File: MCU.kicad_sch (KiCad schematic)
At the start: 14 parts, among them U4 ATSAMD21G18A-A, Y1 ABS07-32.768KHZ-T

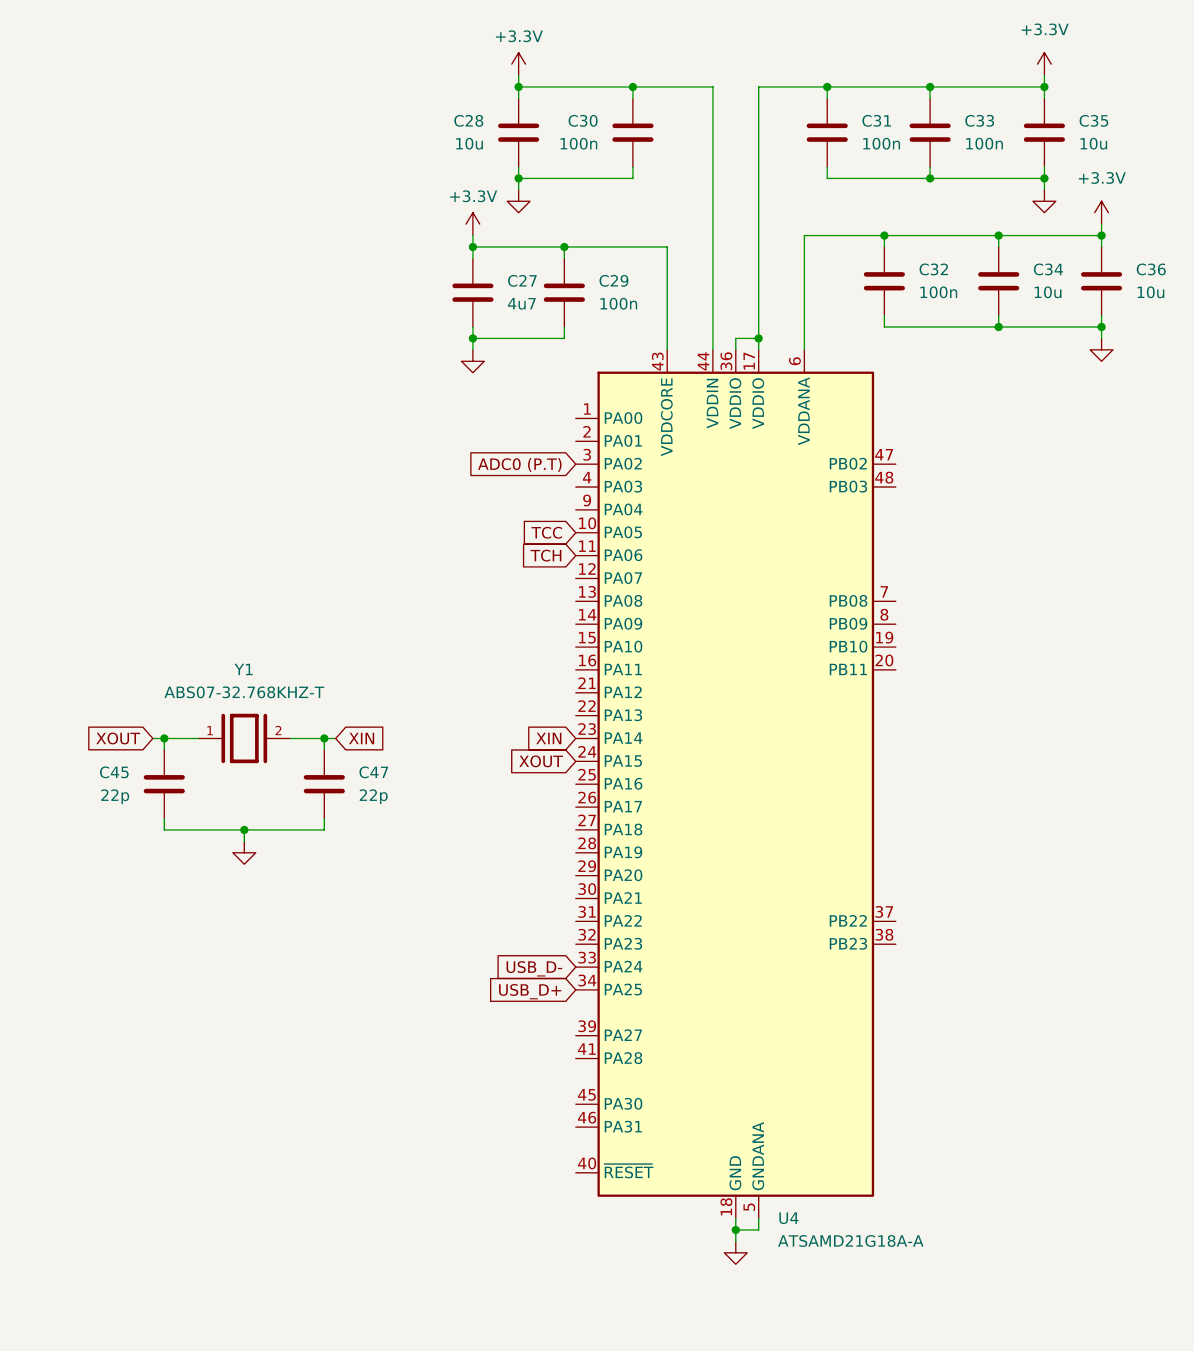
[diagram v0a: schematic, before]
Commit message: Added changes to pass ERC check
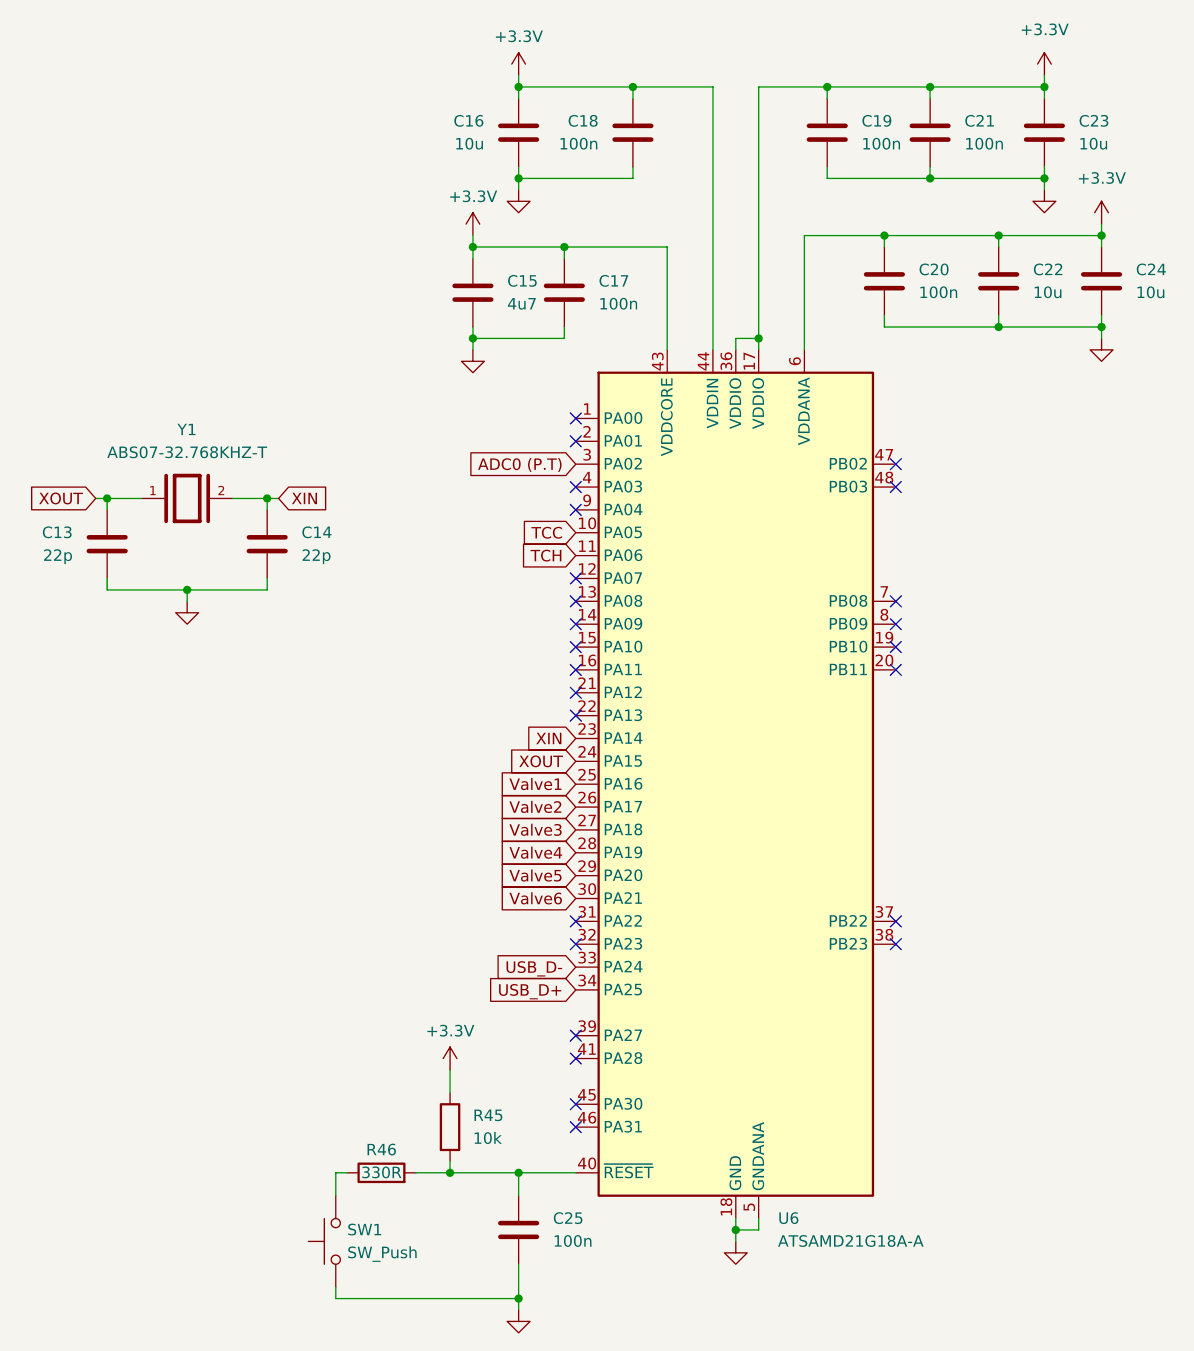
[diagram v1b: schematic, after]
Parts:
- added C25: 100n, symbol Device:C
- added R45: 10k, symbol Device:R
- added R46: 330R, symbol Device:R
- added SW1: SW_Push, Button_Switch_SMD:SW_SPST_B3S-1000, symbol Switch:SW_Push
- renumbered C45 to C13, C47 to C14, C27 to C15, C28 to C16, C29 to C17, C30 to C18, C31 to C19, C32 to C20, C33 to C21, C34 to C22, C35 to C23, C36 to C24, U4 to U6
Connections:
- net +3.3V: now also R45.1
- net GND: now also C25.2, SW1.1
- net Valve1: now reaches U6.25 (PA16)
- net Valve2: now reaches U6.26 (PA17)
- net Valve3: now reaches U6.27 (PA18)
- net Valve4: now reaches U6.28 (PA19)
- net Valve5: now reaches U6.29 (PA20)
- net Valve6: now reaches U6.30 (PA21)
- net at U6.40 (~{RESET}): now also C25.1, R45.2, R46.2
- new net: R46.1, SW1.2
- no-connect marks 0 -> 25
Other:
- moved on the sheet: C13, C14, Y1
